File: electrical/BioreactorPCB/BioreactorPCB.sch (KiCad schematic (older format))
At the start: 56 parts, among them IC1 AL5809-20P1-7, IC2 VEML7700-TR, J1 61300311121, J10 171856-0006, J11 USB_B, J12 Conn_02x03_Odd_Even, J13 Conn_01x05_Male, J2 61300311121, J3 Conn_01x05_Male, J4 PJ-202A, J5 OSTTC022162, J6 OSTTC022162, J7 OSTTC042162, J8 OSTTC042162, J9 OSTTC042162, Q1 2N3905, Q2 IRF540N, Q3 FQP47P06, Q4 TL2575HV-05IKV, U1 FT232RL, U2 L293D, U3 ATMEGA328P-AUR, Y1 16 mHz

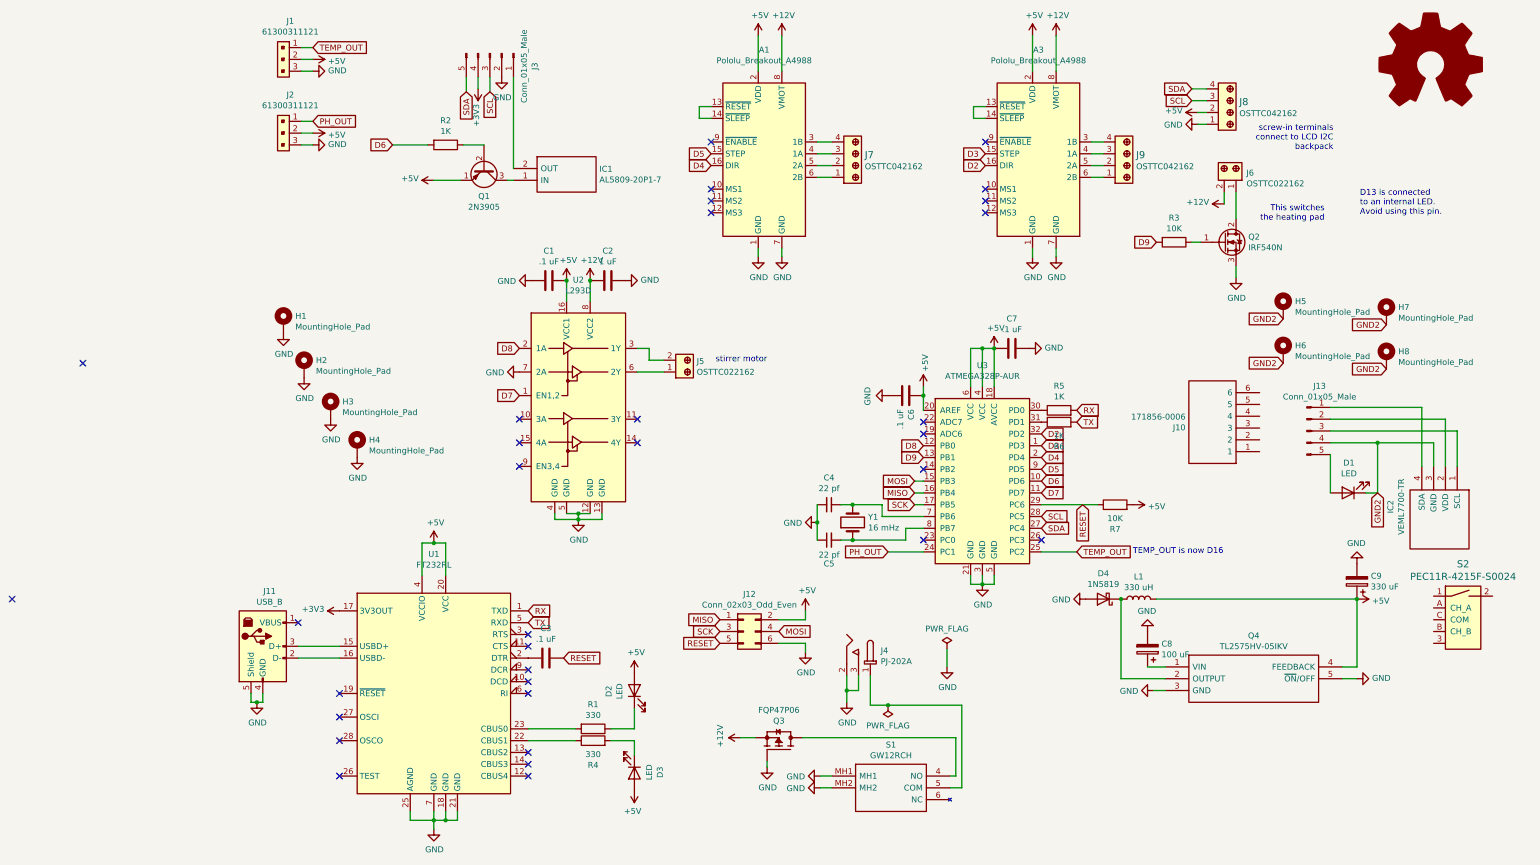
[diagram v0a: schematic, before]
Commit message: Completed rev 2.0 schematic for real now
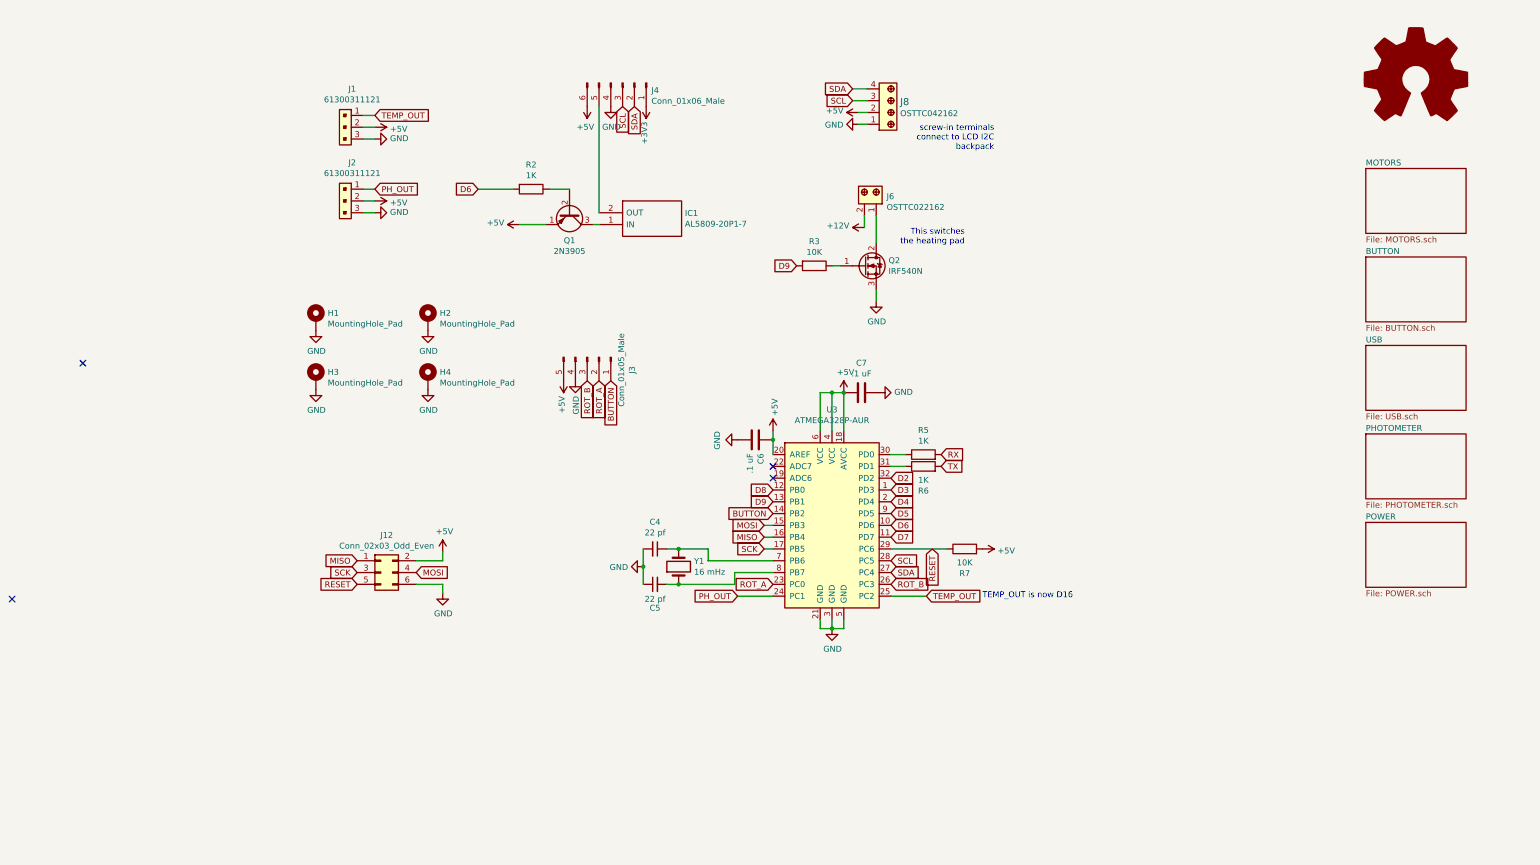
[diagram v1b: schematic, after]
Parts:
- removed A1, A3: Pololu_Breakout_A4988, Module:Pololu_Breakout-16_15.2x20.3mm, symbol Driver_Motor:Pololu_Breakout_A4988
- removed C1, C3: .1 uF, Capacitor_THT:CP_Radial_Tantal_D5.0mm_P2.50mm, symbol Device:C
- removed C2: 1 uF, Capacitor_THT:CP_Radial_Tantal_D5.0mm_P2.50mm, symbol Device:C
- removed C8: 100 uF, Capacitor_THT:CP_Radial_D5.0mm_P2.50mm, symbol Device:CP
- removed C9: 330 uF, Capacitor_THT:CP_Radial_D5.0mm_P2.50mm, symbol Device:CP
- removed D1, D2, D3: LED, LED_THT:LED_D5.0mm_Horizontal_O3.81mm_Z9.0mm, symbol Device:LED
- removed D4: 1N5819, Diode_THT:D_DO-41_SOD81_P10.16mm_Horizontal, symbol Diode:1N5819
- removed H5, H6, H7, H8: MountingHole_Pad, MountingHole:MountingHole_3.2mm_M3_DIN965_Pad, symbol Mechanical:MountingHole_Pad
- removed IC2: VEML7700-TR, VEML7700-TR:VEML7700, symbol VEML7700-TR:VEML7700-TR
- removed J10: 171856-0006, 171856-0006:HDRV6W99P0X254_1X6_1509X635X1100P, symbol 171856-0006:171856-0006
- removed J11: USB_B, Connector_USB:USB_B_Amphenol_MUSB-D511_Vertical_Rugged, symbol Connector:USB_B
- removed J13: Conn_01x05_Male, Connector_Molex:Molex_KK-254_AE-6410-05A_1x05_P2.54mm_Vertical, symbol Connector:Conn_01x05_Male
- removed J4: PJ-202A, digikey-footprints:Barrel_Jack_5.5mmODx2.1mmID_PJ-202A, symbol dk_Barrel-Power-Connectors:PJ-202A
- removed J5: OSTTC022162, digikey-footprints:Term_Block_1x2_P5.08MM, symbol dk_Terminal-Blocks-Wire-to-Board:OSTTC022162
- removed J7, J9: OSTTC042162, digikey-footprints:Term_Block_1x4_P5.08mm, symbol dk_Terminal-Blocks-Wire-to-Board:OSTTC042162
- removed L1: 330 uH, Inductor_THT:L_Radial_D12.0mm_P6.00mm_MuRATA_1900R, symbol Device:L
- removed Q3: FQP47P06, FQP47P06:TO254P1067X483X2286-3, symbol FQP47P06:FQP47P06
- removed Q4: TL2575HV-05IKV, Package_TO_SOT_THT:TO-220-5_P3.4x3.8mm_StaggerEven_Lead7.13mm_TabDown_Heatsink, symbol TL2575HV-05IKV:TL2575HV-05IKV
- removed R1, R4: 330, Resistor_THT:R_Axial_DIN0204_L3.6mm_D1.6mm_P5.08mm_Horizontal, symbol Device:R
- removed S1: GW12RCH, GW12RCH:GW12RCH, symbol GW12RCH:GW12RCH
- removed S2: PEC11R-4215F-S0024, digikey-footprints:Rotary_Encoder_Switched_PEC11R, symbol dk_Encoders:PEC11R-4215F-S0024
- removed U1: FT232RL, Package_SO:SSOP-28_5.3x10.2mm_P0.65mm, symbol Interface_USB:FT232RL
- removed U2: L293D, Package_DIP:DIP-16_W7.62mm, symbol Driver_Motor:L293D
- added J4: Conn_01x06_Male, Connector_Molex:Molex_KK-254_AE-6410-06A_1x06_P2.54mm_Vertical, symbol Connector:Conn_01x06_Male
- J12: footprint Connector_PinHeader_2.54mm:PinHeader_2x03_P2.54mm_Horizontal -> Connector_PinHeader_2.54mm:PinHeader_2x03_P2.54mm_Vertical
- Q2: footprint Package_TO_SOT_THT:TO-220-3_Vertical -> Package_TO_SOT_THT:TO-220-3_Horizontal_TabDown
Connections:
- net +3V3: now also J4.1 (Pin_1); no longer J3.4 (Pin_4)
- net +5V: now also J3.5 (Pin_5), J4.6 (Pin_6)
- net GND: now also J3.4 (Pin_4), J4.4 (Pin_4); no longer J3.2 (Pin_2)
- net SCL: now also J4.3 (Pin_3); no longer J3.3 (Pin_3)
- net SDA: now also J4.2 (Pin_2); no longer J3.5 (Pin_5)
- net at IC1.2 (OUT): now also J4.5 (Pin_5); no longer J3.1 (Pin_1)
- net BUTTON: now reaches U3.14 (PB2)
- net BUTTON: now also J3.1 (Pin_1)
- net ROT_A: now reaches U3.23 (PC0)
- net ROT_A: now also J3.2 (Pin_2)
- net ROT_B: now reaches U3.26 (PC3)
- net ROT_B: now also J3.3 (Pin_3)
- no-connect marks 33 -> 4
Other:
- note removed: "D13 is connected\nto an internal LED.\nAvoid using this pin."
- note removed: "stirrer motor"
- moved on the sheet: C4, C5, C6, C7, H1, H2, H3, H4, IC1, J1, J12, J2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

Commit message: added missing electrolytic capacitors for A4988 breakouts. Preliminary layout now in place
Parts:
- C4, C5: footprint Capacitor_THT:CP_Radial_Tantal_D4.5mm_P2.50mm -> Capacitor_THT:C_Disc_D5.0mm_W2.5mm_P2.50mm
- C6, C7: footprint Capacitor_THT:CP_Radial_Tantal_D5.0mm_P2.50mm -> Capacitor_THT:C_Disc_D5.0mm_W2.5mm_P2.50mm
- Q2: footprint Package_TO_SOT_THT:TO-220-3_Horizontal_TabDown -> Package_TO_SOT_THT:TO-220-3_Vertical
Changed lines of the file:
@@
 F 0 "Q2" H 6054 2796 50  0000 L CNN
 F 1 "IRF540N" H 6054 2705 50  0000 L CNN
-F 2 "Package_TO_SOT_THT:TO-220-3_Horizontal_TabDown" H 6100 2675 50  0001 L CIN
+F 2 "Package_TO_SOT_THT:TO-220-3_Vertical" H 6100 2675 50  0001 L CIN
 F 3 "http://www.irf.com/product-info/datasheets/data/irf540n.pdf" H 5850 2750 50  0001 L CNN
 	1    5850 2750
@@
 F 0 "C6" H 5040 4271 50  0000 L CNN
 F 1 ".1 uF" H 5040 4180 50  0000 L CNN
-F 2 "Capacitor_THT:CP_Radial_Tantal_D5.0mm_P2.50mm" H 4963 4075 50  0001 C CNN
+F 2 "Capacitor_THT:C_Disc_D5.0mm_W2.5mm_P2.50mm" H 4963 4075 50  0001 C CNN
 F 3 "~" H 4925 4225 50  0001 C CNN
 	1    4925 4225
@@
 F 0 "C7" V 5573 3825 50  0000 C CNN
 F 1 ".1 uF" V 5664 3825 50  0000 C CNN
-F 2 "Capacitor_THT:CP_Radial_Tantal_D5.0mm_P2.50mm" H 5863 3675 50  0001 C CNN
+F 2 "Capacitor_THT:C_Disc_D5.0mm_W2.5mm_P2.50mm" H 5863 3675 50  0001 C CNN
 F 3 "~" H 5825 3825 50  0001 C CNN
 	1    5825 3825
@@
 F 0 "C5" V 3875 5450 50  0000 C CNN
 F 1 "22 pf" V 3950 5450 50  0000 C CNN
-F 2 "Capacitor_THT:CP_Radial_Tantal_D4.5mm_P2.50mm" H 4075 5450 50  0001 C CNN
+F 2 "Capacitor_THT:C_Disc_D5.0mm_W2.5mm_P2.50mm" H 4075 5450 50  0001 C CNN
 F 3 "~" H 4075 5450 50  0001 C CNN
 	1    4075 5450
@@
 F 0 "C4" V 3846 5150 50  0000 C CNN
 F 1 "22 pf" V 3937 5150 50  0000 C CNN
-F 2 "Capacitor_THT:CP_Radial_Tantal_D4.5mm_P2.50mm" H 4075 5150 50  0001 C CNN
+F 2 "Capacitor_THT:C_Disc_D5.0mm_W2.5mm_P2.50mm" H 4075 5150 50  0001 C CNN
 F 3 "~" H 4075 5150 50  0001 C CNN
 	1    4075 5150
